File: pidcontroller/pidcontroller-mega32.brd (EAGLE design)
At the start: 101 x 80 mm, 19 parts, among them IC2 MAX3232CWE, IC3 MEGA32-A

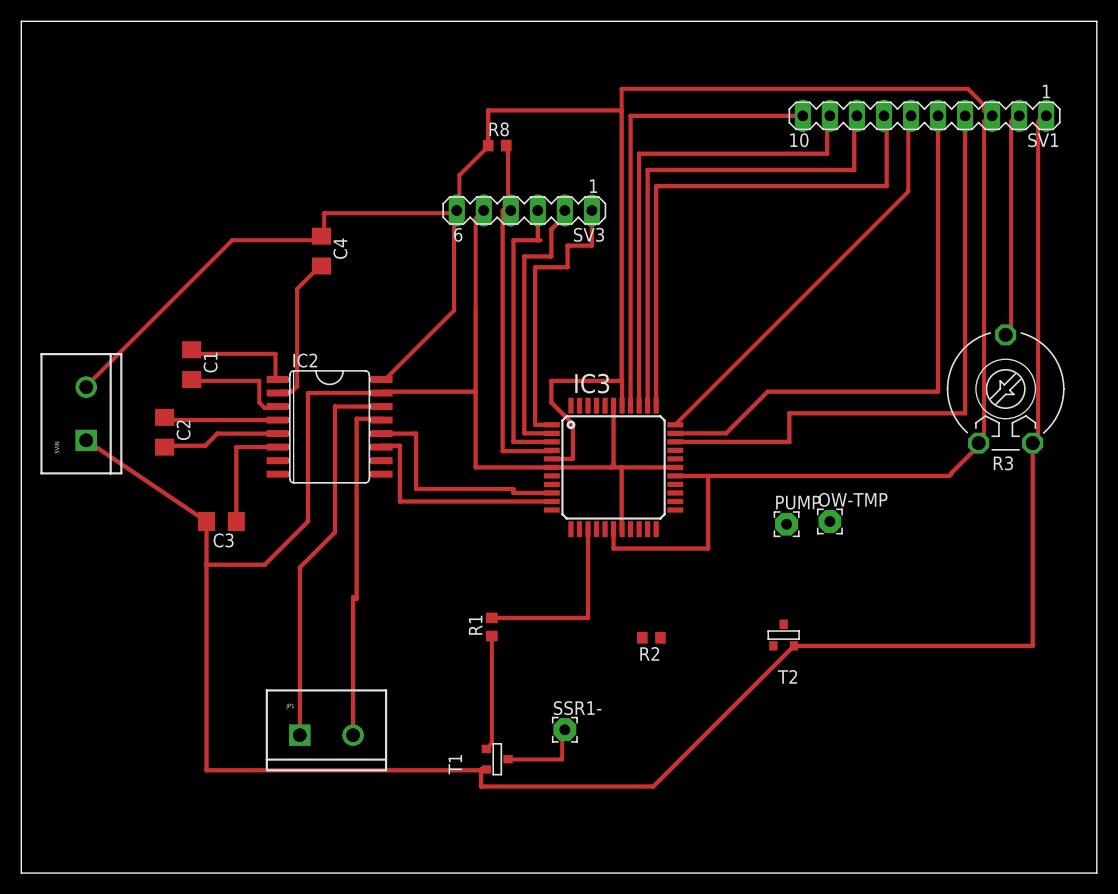
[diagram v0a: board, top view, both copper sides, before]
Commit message: prettified board
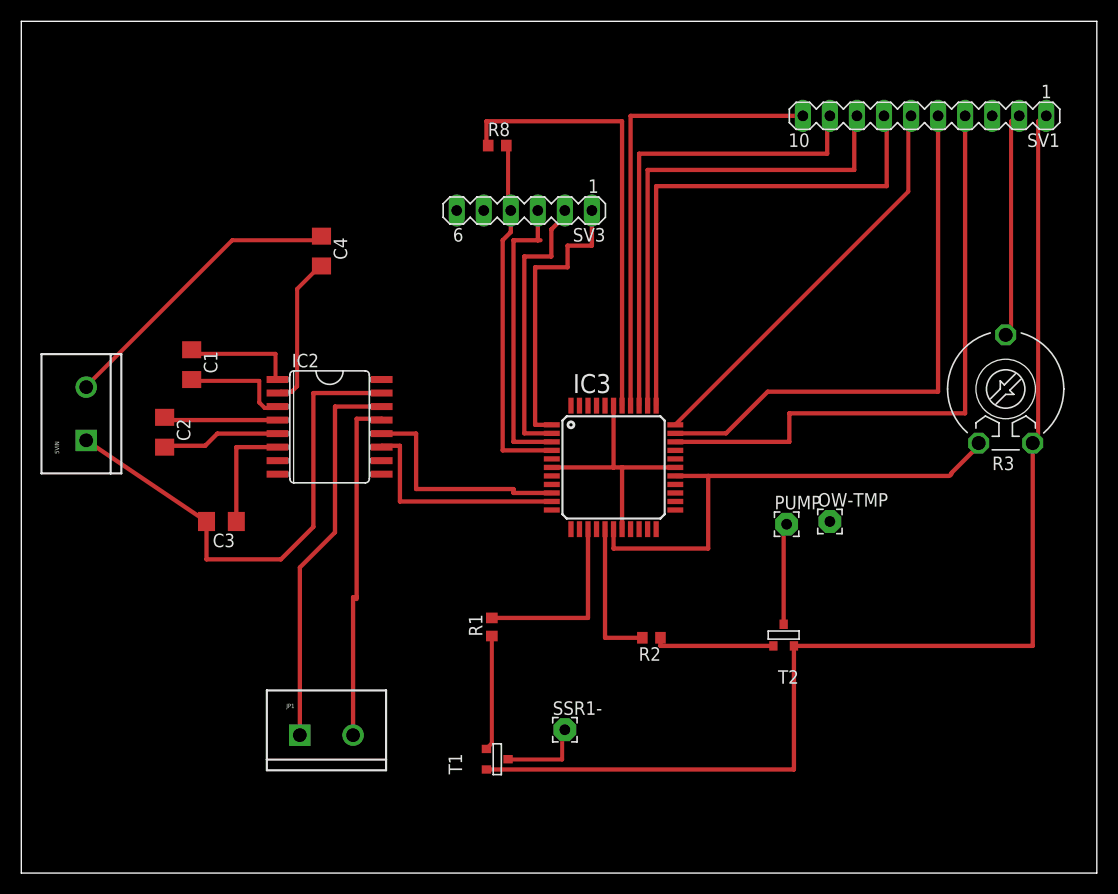
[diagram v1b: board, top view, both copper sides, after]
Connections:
- net GND: now also SV3.6; no longer SV3.5
- net VCC: now also SV3.5; no longer SV3.6
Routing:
- net VCC: track 246.2 -> 117.6 mm
- net GND: track 266.6 -> 184.1 mm
- net N$10: track 0.00 -> 13.7 mm
- net N$3: track 0.00 -> 11.4 mm
- net N$24: track 0.00 -> 9.68 mm
- net RESET: track 34.3 -> 33.7 mm

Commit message: adfasdf
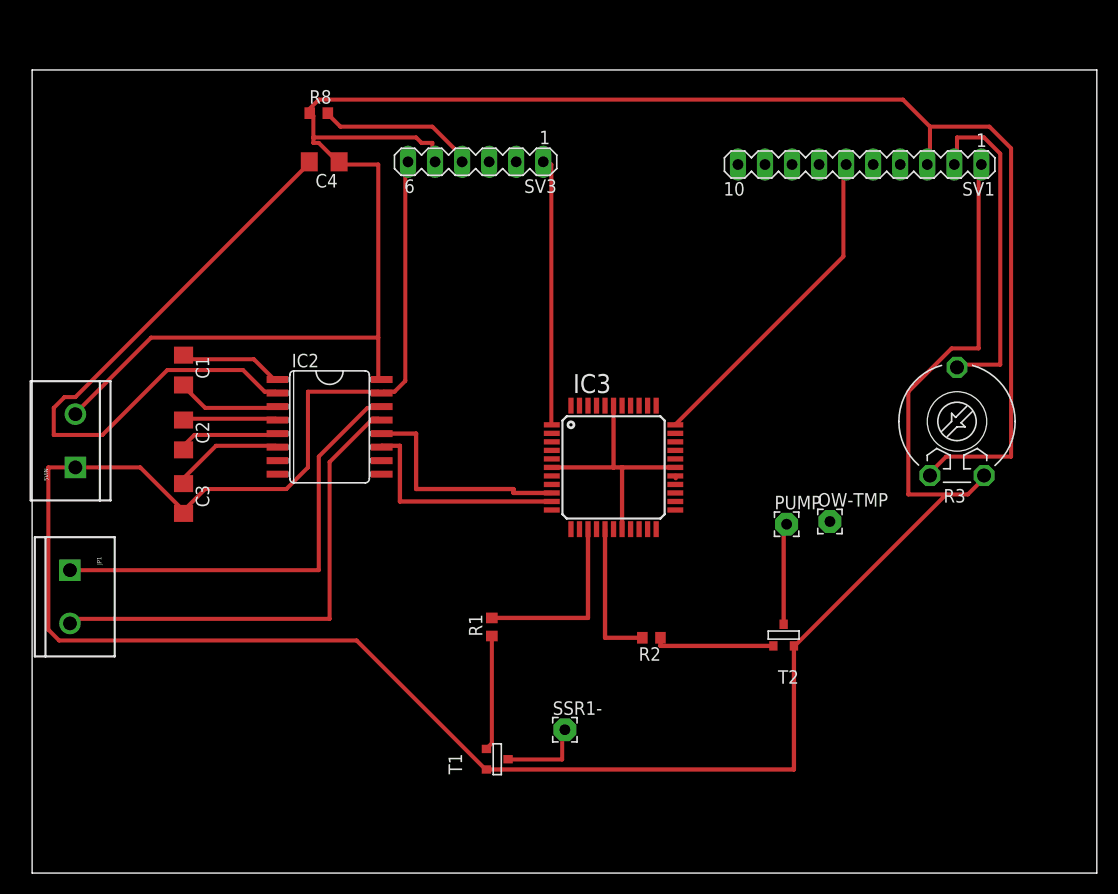
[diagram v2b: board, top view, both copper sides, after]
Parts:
- moved JP1 26.6 mm to (3.56, 28.4), turned to 270 degrees
- moved R8 17.0 mm to (26.9, 71.4)
- moved C4 8.39 mm to (27.4, 66.8), turned to 180 degrees
- moved SV1 7.62 mm to (77.7, 66.5)
- moved SV3 6.47 mm to (41.7, 66.8)
- moved R3 5.49 mm to (86.9, 42.4)
- moved C3 4.16 mm to (14.2, 35.2), turned to 270 degrees
- moved 5VIN 2.74 mm to (4.06, 38.1)
- moved C2 1.80 mm to (14.2, 41.1)
- moved C1 0.92 mm to (14.2, 47.2)
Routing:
- net GND: track 184.1 -> 254.7 mm
- net VCC: track 117.6 -> 185.5 mm
- net D7: track 57.8 -> 0.00 mm
- net D6: track 52.2 -> 0.00 mm
- net D4: track 49.1 -> 0.00 mm
- net E: track 46.9 -> 0.00 mm
- net N$9: track 14.4 -> 60.6 mm
- net RW: track 45.1 -> 0.00 mm
- net RS: track 43.4 -> 0.00 mm
- net N$1: track 27.9 -> 0.00 mm
- net N$15: track 26.6 -> 0.00 mm
- net RESET: track 33.7 -> 15.0 mm
- net 232TX: track 32.7 -> 46.2 mm
- net N$17: track 21.2 -> 31.6 mm
- net D5: track 38.3 -> 31.2 mm
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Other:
- board size 101 x 80 mm -> 100 x 75.4 mm
